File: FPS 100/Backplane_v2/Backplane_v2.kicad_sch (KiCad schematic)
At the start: 69 parts, among them J1 Conn_01x02_Pin, J10 Conn_01x02_Pin, J11 Conn_01x02_Pin, J12 Conn_01x02_Pin, J13 Conn_01x02_Pin, J14 Conn_01x02_Pin, J15 Conn_01x02_Pin, J16 Conn_01x02_Pin, J17 Conn_01x02_Pin, J18 Conn_01x02_Pin, J19 Conn_01x02_Pin, J2 Conn_01x02_Pin, J20 Conn_01x02_Pin, J21 Conn_01x02_Pin, J22 Conn_01x02_Pin, J23 Conn_01x02_Pin, J24 Conn_01x02_Pin, J25 Conn_01x02_Pin, J26 Conn_01x02_Pin, J27 Conn_01x02_Pin, J28 Conn_01x02_Pin, J29 Conn_01x02_Pin, J3 Conn_01x02_Pin, J30 Conn_01x02_Pin, J31 Conn_01x02_Pin, J32 Conn_01x02_Pin, J33 Conn_01x02_Pin, J34 Conn_01x02_Pin, J35 Conn_01x02_Pin, J36 Conn_01x02_Pin, J37 Conn_01x02_Pin, J38 Conn_01x02_Pin, J39 Indicator Panel, J4 Conn_01x02_Pin, J40 Conn_01x02_Pin, J41 Conn_01x02_Pin, J6 Conn_01x02_Pin, J7 Conn_01x02_Pin, J8 Conn_01x02_Pin, J9 Conn_01x02_Pin

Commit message: 2026/1/21
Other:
- note added: "These are NOT etched Use external twisted pair wires !SPCLK P3.A.005 <-> P1.A.006 !WRT* P3.A.006 <-> P1.A.005 <-> P2.A.006 !CBCLK2 P3.A.007 <-> P2.A.005 !CBCLK1 P3.A.008 <-> P1.A.007 !WRTR* P3.A.009 <-> DPR.A.006 !TMCLK P3.A.010 <-> TM.A.005 !T75 P3.A.011 <-> MD.A.006 !MICLK P3.A.012 <-> FM.A.005 !FMCLK P3.A.013 <-> FM.A.006 !A2CLK P3.A.014 <-> FA.A.010 <-> FM.A.010 !A1CLK P3.A.015 <-> FA.A.008 <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"
- note removed: "!SPCLK P3.A.005 <-> P1.A.006 !WRT* P3.A.006 <-> P1.A.005 <-> P2.A.006 !CBCLK2 P3.A.007 <-> P2.A.005 !CBCLK1 P3.A.008 <-> P1.A.007 !WRTR* P3.A.009 <-> DPR.A.006 !TMCLK P3.A.010 <-> TM.A.005 !T75 P3.A.011 <-> MD.A.006 !MICLK P3.A.012 <-> FM.A.005 !FMCLK P3.A.013 <-> FM.A.006 !A2CLK P3.A.014 <-> FA.A.010 <-> FM.A.010 !A1CLK P3.A.015 <-> FA.A.008 <-> FM.A.008 !DPLCLK P3.A.016 <-> DPL.A.005 !DPRCLK P3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"
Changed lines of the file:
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@@
 		)
 	)
-	(text "!SPCLK      P3.A.005 <->  P1.A.006\n!WRT*       P3.A.006 <->  P1.A.005 <-> P2.A.006\n!CBCLK2     P3.A.007 <->  P2.A.005\n!CBCLK1     P3.A.008 <->  P1.A.007\n!WRTR*      P3.A.009 <-> DPR.A.006\n!TMCLK      P3.A.010 <->  TM.A.005\n!T75        P3.A.011 <->  MD.A.006\n!MICLK      P3.A.012 <->  FM.A.005\n!FMCLK      P3.A.013 <->  FM.A.006\n!A2CLK      P3.A.014 <->  FA.A.010 <-> FM.A.010\n!A1CLK      P3.A.015 <->  FA.A.008 <-> FM.A.008\n!DPLCLK     P3.A.016 <-> DPL.A.005\n!DPRCLK     P3.A.017 <-> DPR.A.005\n!WRTL*      P3.A.018 <-> DPL.A.006\n!FACLK      P3.A.019 <->  FA.A.006\n!IOCLK      P3.A.020 <->  IF.A.006\n!MCLK       P3.A.021 <->  MD.A.005\n!HRSET*     P3.A.025 <->  IF.B.052\nEXTCLK{408} P3.B.115 <-> External Clock (if jumpered)"
+	(text "These are NOT etched\nUse external twisted pair wires\n\n!SPCLK      P3.A.005 <->  P1.A.006\n!WRT*       P3.A.006 <->  P1.A.005 <-> P2.A.006\n!CBCLK2     P3.A.007 <->  P2.A.005\n!CBCLK1     P3.A.008 <->  P1.A.007\n!WRTR*      P3.A.009 <-> DPR.A.006\n!TMCLK      P3.A.010 <->  TM.A.005\n!T75        P3.A.011 <->  MD.A.006\n!MICLK      P3.A.012 <->  FM.A.005\n!FMCLK      P3.A.013 <->  FM.A.006\n!A2CLK      P3.A.014 <->  FA.A.010 <-> FM.A.010\n!A1CLK      P3.A.015 <->  FA.A.008 <-> FM.A.008\n!DPLCLK     P3.A.016 <-> DPL.A.005\n!DPRCLK     P3.A.017 <-> DPR.A.005\n!WRTL*      P3.A.018 <-> DPL.A.006\n!FACLK      P3.A.019 <->  FA.A.006\n!IOCLK      P3.A.020 <->  IF.A.006\n!MCLK       P3.A.021 <->  MD.A.005\n!HRSET*     P3.A.025 <->  IF.B.052\nEXTCLK{408} P3.B.115 <-> External Clock (if jumpered)"
 		(exclude_from_sim no)
-		(at 708.914 444.246 0)
+		(at 707.898 460.502 0)
 		(effects
 			(font
@@
 	(wire
 		(pts
+			(xy 664.21 367.03) (xy 643.89 367.03)
+		)
+		(stroke
+			(width 0)
+			(type default)
+		)
+	)
+	(wire
+		(pts
 			(xy 963.93 455.93) (xy 963.93 458.47)
 		)
@@
 	(wire
 		(pts
+			(xy 523.24 90.17) (xy 549.91 90.17)
+		)
+		(stroke
+			(width 0)
+			(type default)
+		)
+	)
+	(wire
+		(pts
 			(xy 923.29 420.37) (xy 923.29 422.91)
 		)
@@
 	(global_label "RBUEQ*"
 		(shape input)
-		(at 643.89 367.03 0)
+		(at 664.21 367.03 0)
 		(fields_autoplaced yes)
 		(effects
@@
 		)
 		(property "Intersheetrefs" "${INTERSHEET_REFS}"
-			(at 654.1928 367.03 0)
+			(at 674.5128 367.03 0)
 			(effects
 				(font
@@
 	(global_label "RBUFQ"
 		(shape input)
-		(at 549.91 90.17 180)
+		(at 523.24 90.17 180)
 		(fields_autoplaced yes)
 		(effects
@@
 		)
 		(property "Intersheetrefs" "${INTERSHEET_REFS}"
-			(at 540.6352 90.17 0)
+			(at 513.9652 90.17 0)
 			(effects
 				(font

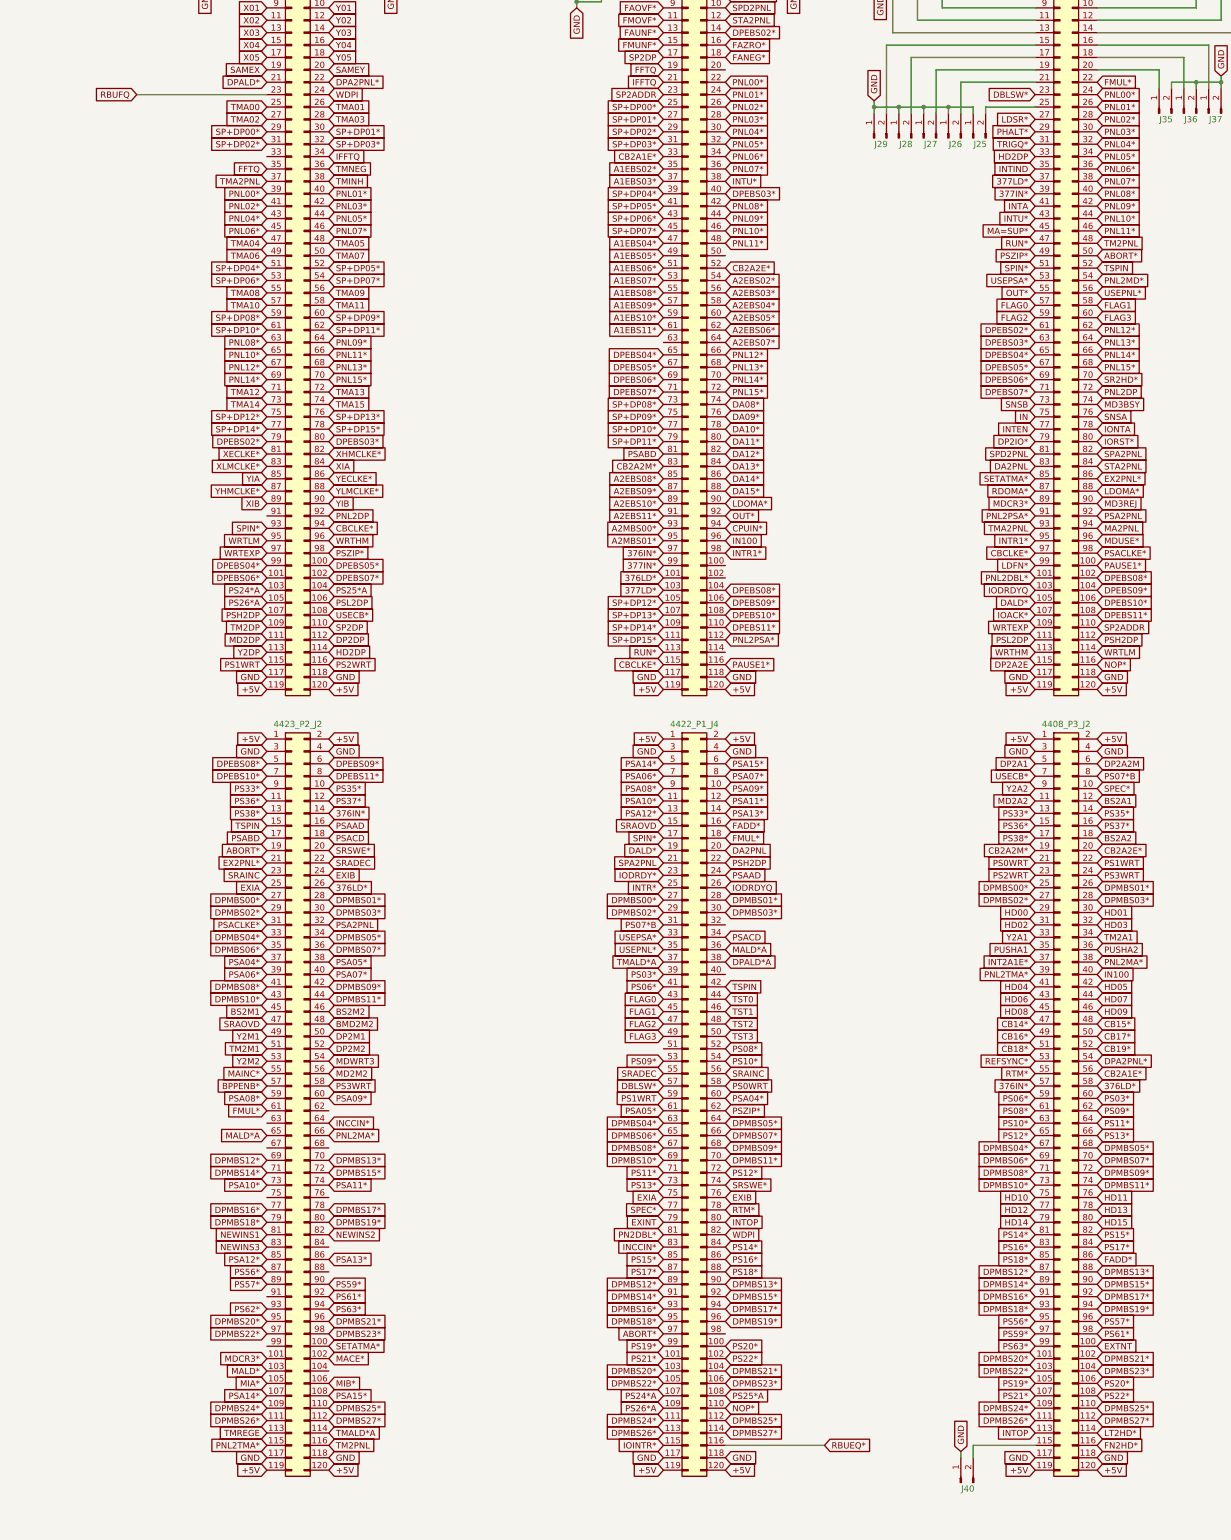
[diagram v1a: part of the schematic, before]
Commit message: 2026/1/26
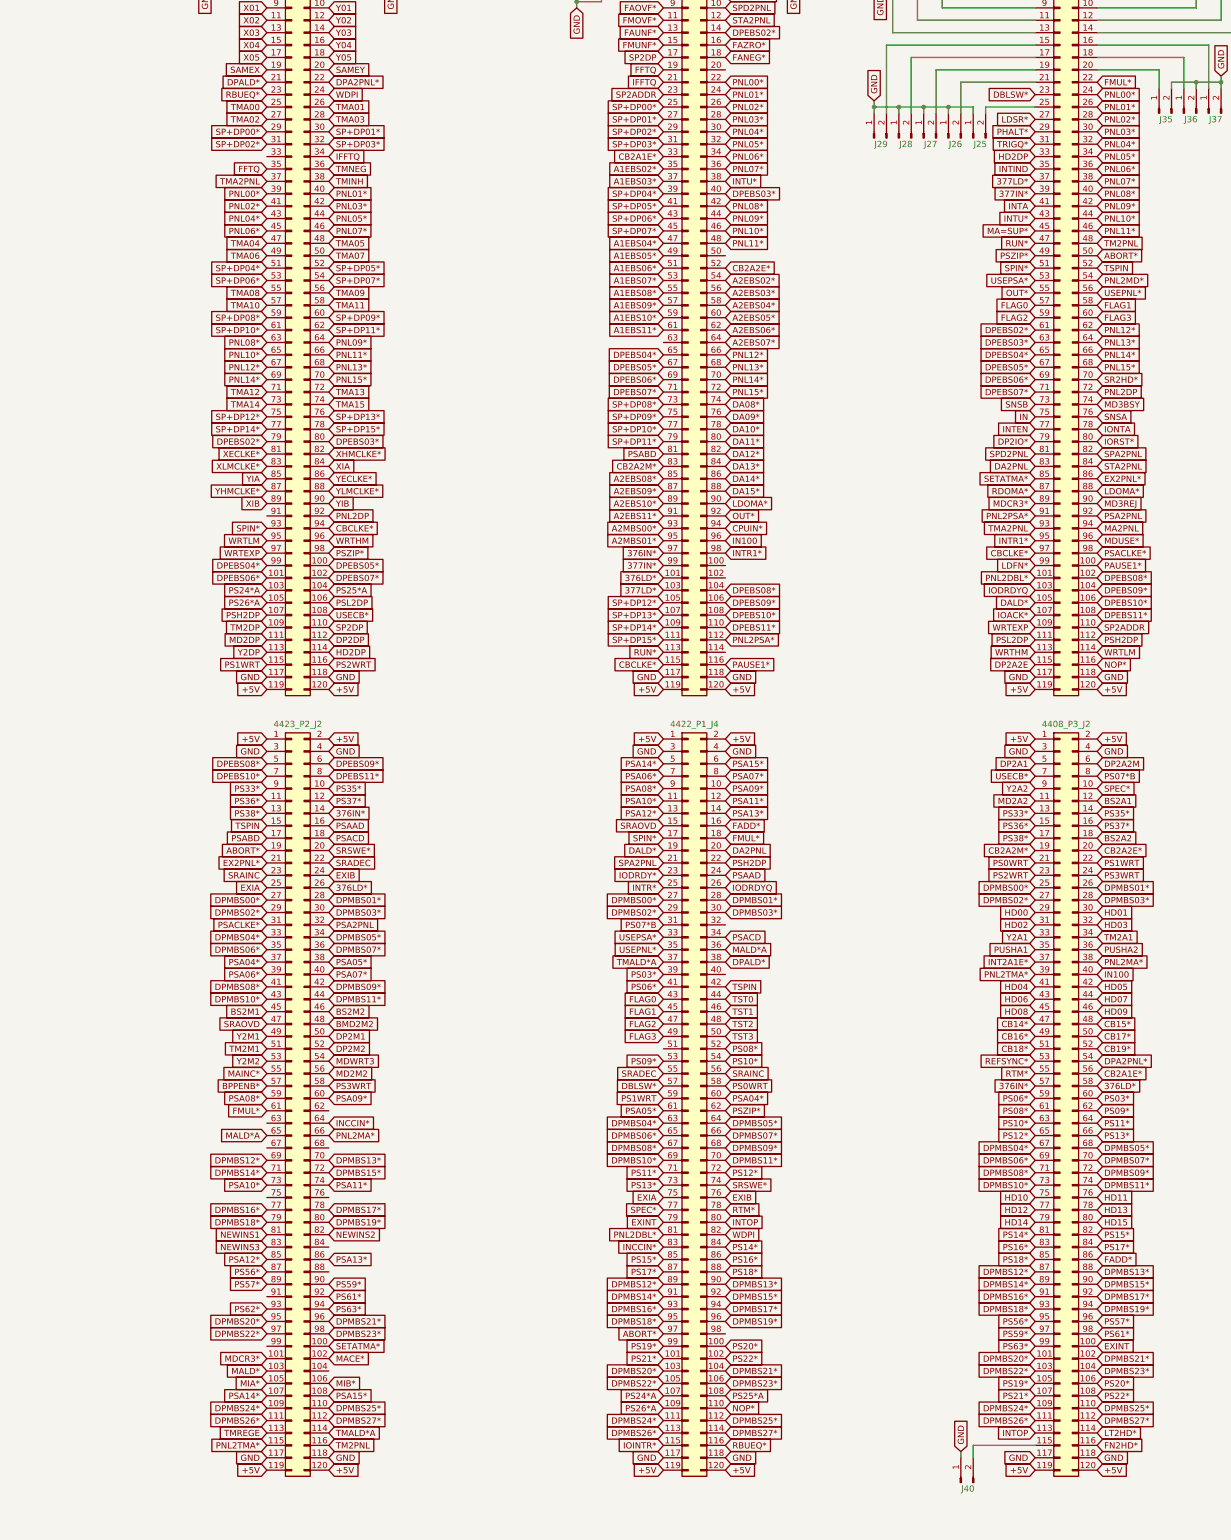
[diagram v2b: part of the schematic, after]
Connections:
- net DPALD*A is gone; now on net DPALD*: 4422_P1_J4.38
- net EXTNT is gone; now on net EXINT: 4408_P3_J2.100
- net PN2DBL* is gone; now on net PNL2DBL*: 4422_P1_J4.81
- net RBUFQ is gone; now on net RBUEQ*: 4423_P2_J1.23
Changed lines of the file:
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@@
 	(wire
 		(pts
-			(xy 664.21 367.03) (xy 643.89 367.03)
-		)
-		(stroke
-			(width 0)
-			(type default)
-		)
-	)
-	(wire
-		(pts
 			(xy 963.93 455.93) (xy 963.93 458.47)
 		)
@@
 	(wire
 		(pts
-			(xy 523.24 90.17) (xy 549.91 90.17)
-		)
-		(stroke
-			(width 0)
-			(type default)
-		)
-	)
-	(wire
-		(pts
 			(xy 923.29 420.37) (xy 923.29 422.91)
 		)
@@
 	(global_label "RBUEQ*"
 		(shape input)
-		(at 664.21 367.03 0)
+		(at 643.89 367.03 0)
 		(fields_autoplaced yes)
 		(effects
@@
 		)
 		(property "Intersheetrefs" "${INTERSHEET_REFS}"
-			(at 674.5128 367.03 0)
+			(at 654.1928 367.03 0)
 			(effects
 				(font
@@
 		)
 	)
-	(global_label "PN2DBL*"
+	(global_label "PNL2DBL*"
 		(shape input)
 		(at 631.19 323.85 180)
@@
 		)
 		(property "Intersheetrefs" "${INTERSHEET_REFS}"
-			(at 619.8591 323.85 0)
+			(at 618.831 323.85 0)
 			(effects
 				(font
@@
 		)
 	)
-	(global_label "RBUFQ"
+	(global_label "RBUEQ*"
 		(shape input)
-		(at 523.24 90.17 180)
+		(at 549.91 90.17 180)
 		(fields_autoplaced yes)
 		(effects
@@
 		)
 		(property "Intersheetrefs" "${INTERSHEET_REFS}"
-			(at 513.9652 90.17 0)
+			(at 539.6072 90.17 0)
 			(effects
 				(font
@@
 		)
 	)
-	(global_label "DPALD*A"
+	(global_label "DPALD*"
 		(shape input)
 		(at 643.89 267.97 0)
@@
 		)
 		(property "Intersheetrefs" "${INTERSHEET_REFS}"
-			(at 654.8581 267.97 0)
+			(at 653.7695 267.97 0)
 			(effects
 				(font
@@
 		)
 	)
-	(global_label "EXTNT"
+	(global_label "EXINT"
 		(shape input)
 		(at 720.09 346.71 0)
@@
 		)
 		(property "Intersheetrefs" "${INTERSHEET_REFS}"
-			(at 728.6994 346.71 0)
+			(at 728.3366 346.71 0)
 			(effects
 				(font
